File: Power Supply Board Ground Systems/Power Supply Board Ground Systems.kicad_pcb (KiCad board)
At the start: 2 copper layers, 114.3 x 50.8 mm, 22 parts, among them J1 POWER, J2 POWER OUT, SW1 SW_DIP_x01, SW2 SW_DIP_x01, SW3 SW_DIP_x01, SW4 SW_DIP_x01

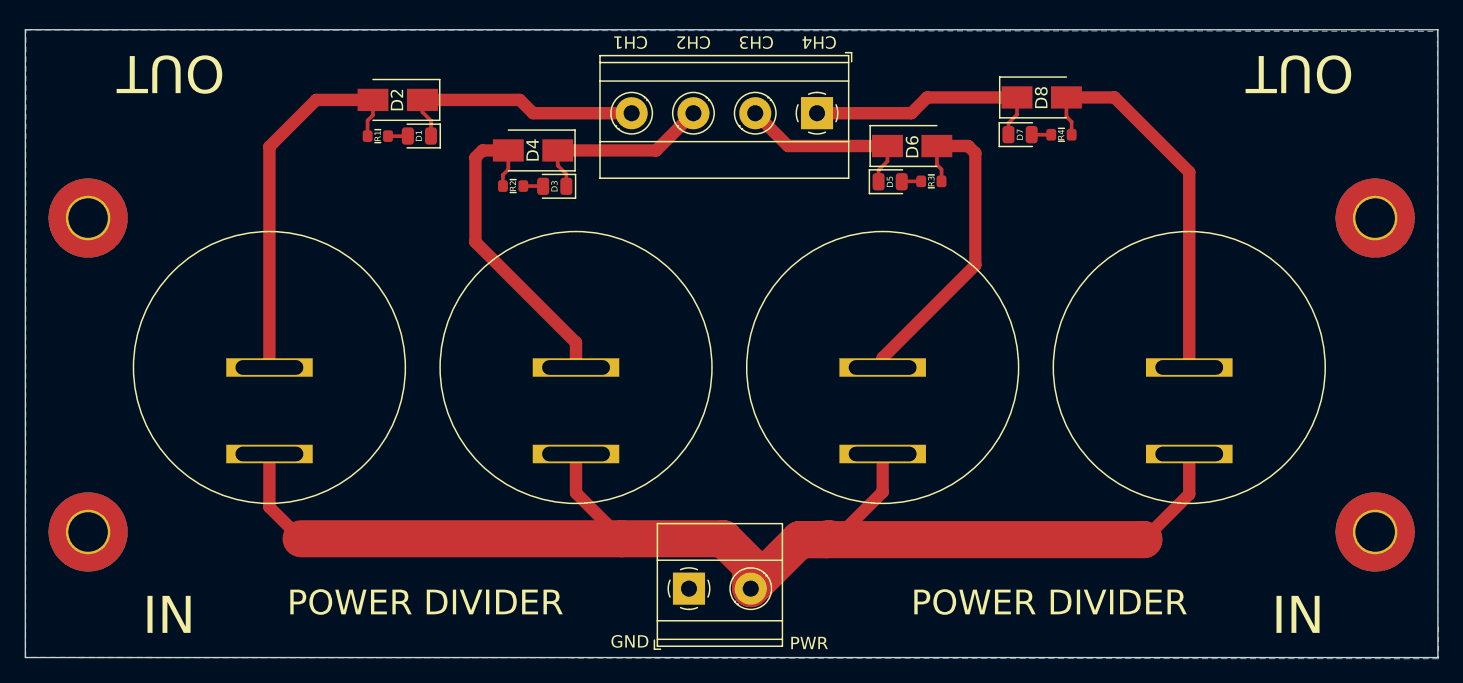
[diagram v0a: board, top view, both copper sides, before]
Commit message: Idk lol some format changes
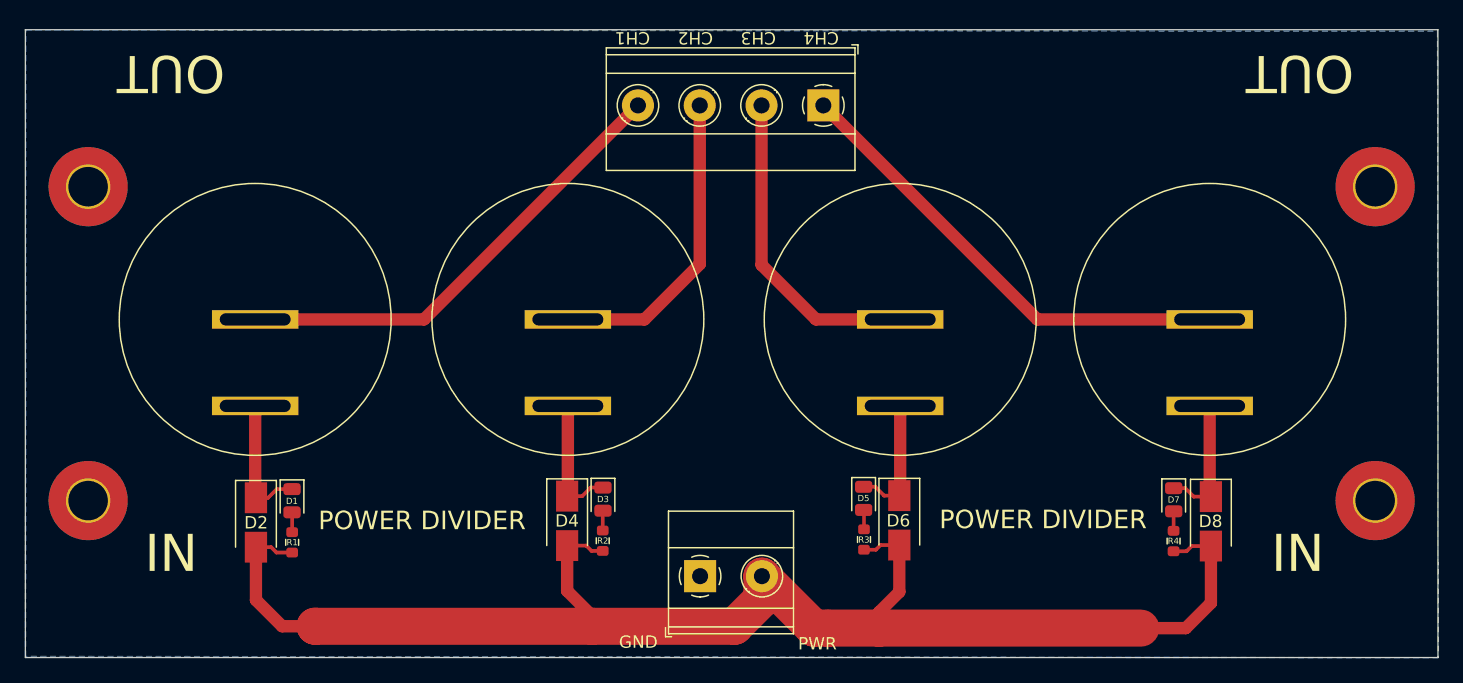
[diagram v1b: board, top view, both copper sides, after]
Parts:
- moved D8 36.9 mm to (121.3, 65.2), turned to -90 degrees
- moved D2 36.1 mm to (44.1, 65.3), turned to -90 degrees
- moved R4 34.1 mm to (118.3, 66.8), turned to -90 degrees
- moved R1 33.6 mm to (47.0, 66.9), turned to -90 degrees
- moved D7 32.0 mm to (118.3, 63.4), turned to -90 degrees
- moved D1 31.3 mm to (47.0, 63.5), turned to -90 degrees
- moved D6 30.3 mm to (96.1, 65.1), turned to -90 degrees
- moved D4 30.1 mm to (69.2, 65.1), turned to -90 degrees
- moved R2 29.6 mm to (72.1, 66.8), turned to -90 degrees
- moved R3 29.5 mm to (93.3, 66.7), turned to -90 degrees
- moved D5 25.7 mm to (93.2, 63.3), turned to -90 degrees
- moved D3 25.6 mm to (72.1, 63.4), turned to -90 degrees
- moved SW4 4.23 mm to (121.2, 48.8)
- moved SW3 4.14 mm to (96.2, 48.8)
- moved SW1 4.06 mm to (44.0, 48.8)
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- renumbered H3 to Hw
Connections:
- D1 pad 1: OUT1 -> PSW1
- D2 pad 1: OUT1 -> PSW1
- D2 pad 2: PSW1 -> POW IN
- D3 pad 1: OUT2 -> PSW2
- D4 pad 1: OUT2 -> PSW2
- D4 pad 2: PSW2 -> POW IN
- D5 pad 1: OUT3 -> PSW3
- D6 pad 1: OUT3 -> PSW3
- D6 pad 2: PSW3 -> POW IN
- D7 pad 1: OUT4 -> PSW4
- D8 pad 1: OUT4 -> PSW4
- D8 pad 2: PSW4 -> POW IN
- R1 pad 2: PSW1 -> POW IN
- R2 pad 2: PSW2 -> POW IN
- R3 pad 2: PSW3 -> POW IN
- R4 pad 2: PSW4 -> POW IN
- SW1 pad 1: POW IN -> PSW1
- SW1 pad 2: PSW1 -> OUT1
- SW2 pad 1: POW IN -> PSW2
- SW2 pad 2: PSW2 -> OUT2
- SW3 pad 1: POW IN -> PSW3
- SW3 pad 2: PSW3 -> OUT3
- SW4 pad 1: POW IN -> PSW4
- SW4 pad 2: PSW4 -> OUT4
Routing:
- net PSW4: track 31.4 -> 10.9 mm
- net PSW1: track 30.9 -> 10.8 mm
- net OUT4: track 20.0 -> 38.4 mm
- net OUT1: track 20.6 -> 38.1 mm
- net PSW3: track 26.8 -> 10.5 mm
- net PSW2: track 26.3 -> 10.5 mm
- net OUT3: track 15.0 -> 26.0 mm
- net POW IN: track 108.9 -> 119.5 mm
- net OUT2: track 15.4 -> 25.4 mm
